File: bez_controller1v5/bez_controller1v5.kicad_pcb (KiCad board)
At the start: 4 copper layers, 100 x 60 mm, 80 parts, among them J1 Conn_01x03_Male, J10 Conn_01x07_Socket, J11 Conn_01x03_Male, J12 Conn_01x03_Male, J13 USB_B_Mini, J14 JTAG Conn_01x06_Male, J15 IMU Conn_01x08_Female, J2 Conn_01x03_Male, J3 Conn_01x03_Male, J4 Screw_Terminal_01x02, J5 Conn_01x03_Male, J6 Conn_01x03_Male, J7 Conn_01x03_Male, J8 JTAG Conn_01x06_Male, J9 Conn_01x09_Socket, U1 PX07806-500-S, U10 USBLC6-4SC6, U11 74LVC2G241, U12 74LVC2G241, U2 74LVC2G241, U3 74LVC2G241, U4 LF50ABV_TO220, U5 LD1117AS33TR_SOT223, U6 INA180A1, U7 STM32F446RETx, U8 74LVC2G241, U9 74LVC2G241, Y1 8MHz

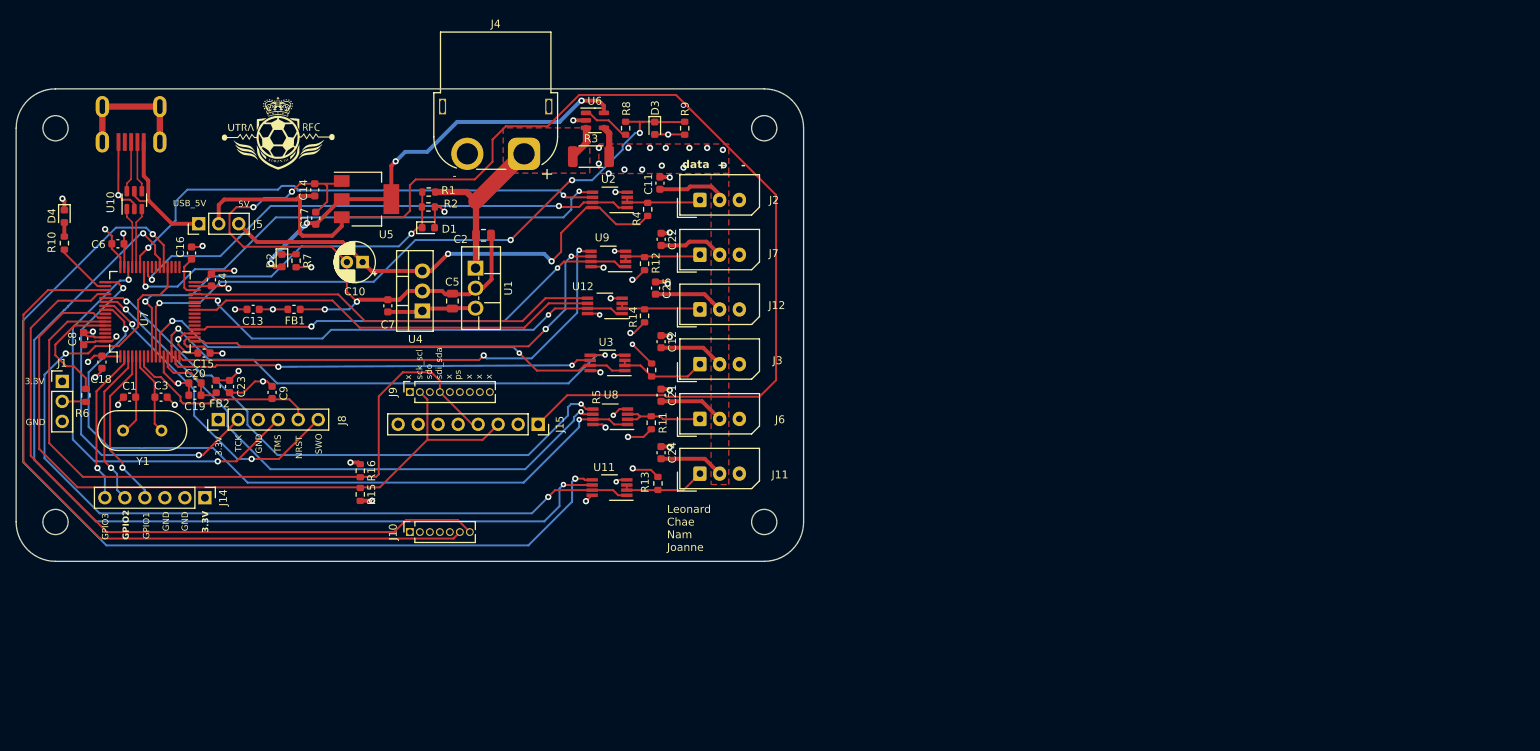
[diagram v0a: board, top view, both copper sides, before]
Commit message: First iteration of the new board with new functions
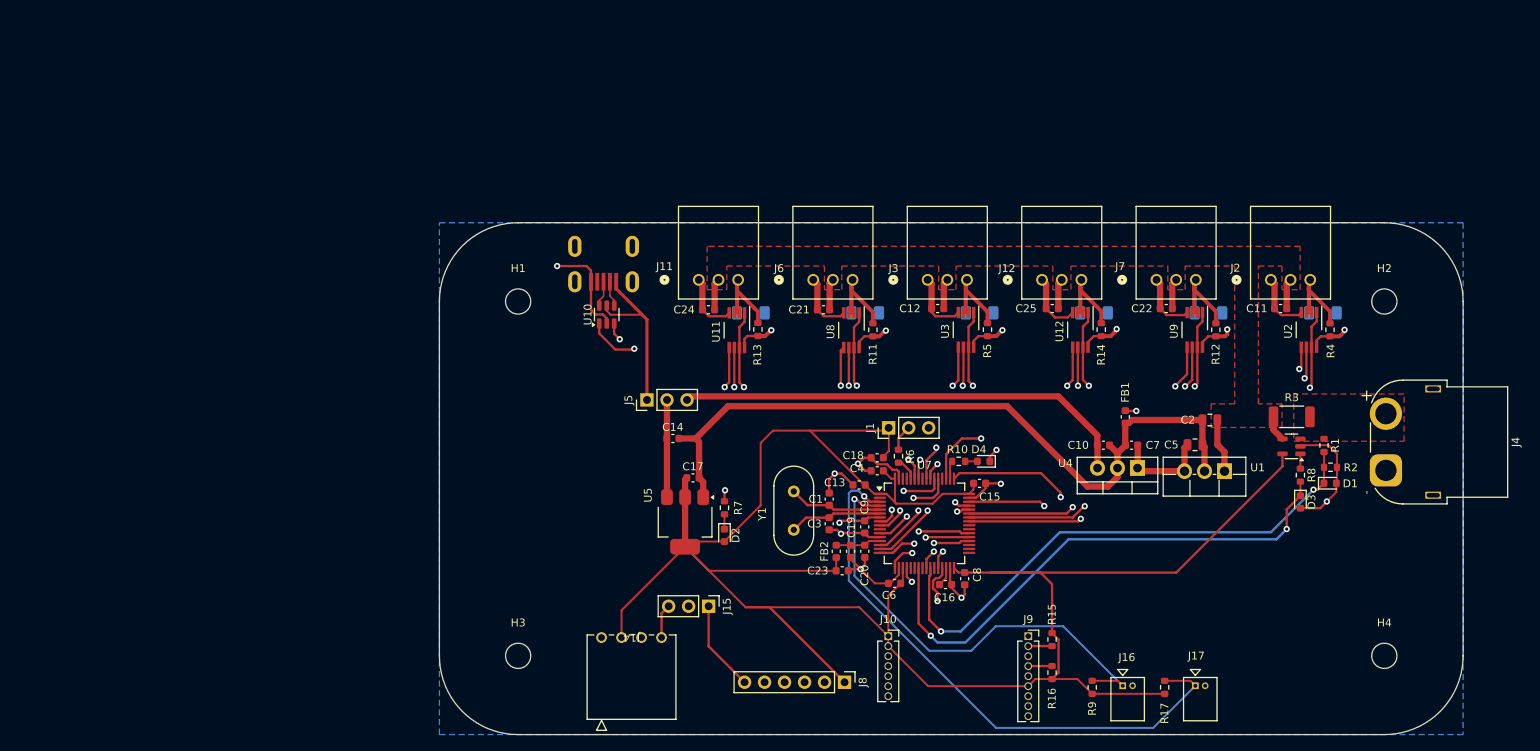
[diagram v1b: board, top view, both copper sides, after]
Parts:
- removed G***: LOGO, LOGO
- added D10: BZV55B5V1, Diode_SMD:D_MiniMELF, B.Cu at (181.4, 54.5)
- added D5: BZV55B5V1, Diode_SMD:D_MiniMELF, B.Cu at (166.9, 54.5)
- added D6: BZV55B5V1, Diode_SMD:D_MiniMELF, B.Cu at (123.3, 54.5)
- added D7: BZV55B5V1, Diode_SMD:D_MiniMELF, B.Cu at (195.9, 54.5)
- added D8: BZV55B5V1, Diode_SMD:D_MiniMELF, B.Cu at (137.8, 54.5)
- added D9: BZV55B5V1, Diode_SMD:D_MiniMELF, B.Cu at (152.3, 54.5)
- added J16: MOLEX_Conn_Button, KiCad:CON_530480210_MOL, F.Cu at (170.5, 101.8)
- added J17: MOLEX_Conn_Button, KiCad:CON_530480210_MOL, F.Cu at (179.8, 101.8)
- added R17: 1k, Resistor_SMD:R_0603_1608Metric, F.Cu at (175.8, 102.0)
- C10: footprint Capacitor_THT:CP_Radial_D5.0mm_P2.00mm -> Capacitor_SMD:C_0603_1608Metric
- J11, J12, J2, J3, J6, J7: footprint Connector_Molex:Molex_SPOX_5267-03A_1x03_P2.50mm_Vertical -> KiCad:CONN_S3B-XH-ALFSN_JST
- J13: footprint USB-Library:USB_MINI -> KiCad:USB_MINI
- J14: value JTAG Conn_01x06_Male -> PPTC041LGBN-RC; footprint Connector_PinHeader_2.54mm:PinHeader_1x06_P2.54mm_Vertical -> KiCad:CONN_PPTC041LGBN-RC_SUL
- J15: value IMU Conn_01x08_Female -> Conn_01x03_Male; footprint Connector_PinSocket_2.54mm:PinSocket_1x08_P2.54mm_Vertical -> Connector_PinHeader_2.54mm:PinHeader_1x03_P2.54mm_Vertical
- R3: value 5m -> 10m
- R9: value 10k -> 1k
- U11, U12, U2, U3, U8, U9: footprint Package_SO:VSSOP-8_3.0x3.0mm_P0.65mm -> KiCad:VSSOP-8_3.0x3.0mm_P0.65mm
- moved H2 170.2 mm to (203.8, 53.0)
- moved D4 120.8 mm to (152.9, 73.3), turned to 180 degrees
- moved R2 119.2 mm to (196.9, 74.0)
- moved D1 119.0 mm to (196.9, 76.1)
- moved R1 118.2 mm to (196.1, 71.3), turned to -90 degrees
- moved R10 116.9 mm to (149.7, 73.3), turned to 180 degrees
- moved J4 116.6 mm to (203.9, 74.5), turned to -90 degrees
- moved C8 116.0 mm to (150.4, 88.2), turned to -90 degrees
- moved C6 107.6 mm to (141.6, 88.8), turned to 180 degrees
- moved FB1 106.4 mm to (170.8, 67.7), turned to -90 degrees
- moved J1 105.1 mm to (140.8, 69.0), turned to 90 degrees
- moved C16 104.6 mm to (148.0, 89.0), turned to 0 degrees
- moved R6 103.5 mm to (142.1, 72.7), turned to -90 degrees
- moved H4 103.4 mm to (203.8, 98.0)
- moved U7 102.0 mm to (145.3, 81.2), turned to 0 degrees
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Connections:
- C11 pad 2: +12V -> /post_shunt_12v
- C12 pad 2: +12V -> /post_shunt_12v
- C2 pad 1: +12V -> /post_shunt_12v
- C21 pad 2: +12V -> /post_shunt_12v
- C22 pad 2: +12V -> /post_shunt_12v
- C24 pad 2: +12V -> /post_shunt_12v
- C25 pad 2: +12V -> /post_shunt_12v
- J11 pad 2: +12V -> /post_shunt_12v
- J12 pad 2: +12V -> /post_shunt_12v
- J14 pad 1: +3.3V -> GND
- J14 pad 2: GND -> +3.3V
- J14 pad 3: GND -> /Screen_SCL
- J14 pad 4: /GPIO1 -> /Screen_SDA
- J15 pad 1: /power -> /SWO
- J15 pad 2: GND -> /SWO_or_Screen_SDA
- J15 pad 3: /SCK_SCL -> /Screen_SDA
- J2 pad 2: +12V -> /post_shunt_12v
- J3 pad 2: +12V -> /post_shunt_12v
- J6 pad 2: +12V -> /post_shunt_12v
- J7 pad 2: +12V -> /post_shunt_12v
- R3 pad 2: +12V -> /post_shunt_12v
- R9 pad 1: /V_shunt_read -> +3.3V
- R9 pad 2: GND -> /GPIO1
- U1 pad 1: +12V -> /post_shunt_12v
- U6 pad 4: +12V -> /post_shunt_12v
- U7 pad 10: /V_shunt_read -> unconnected-(U7-PC2-Pad10)
- U7 pad 2: /GPIO3 -> unconnected-(U7-PC13-Pad2)
- U7 pad 23: unconnected-(U7-PA7-Pad23) -> /V_shunt_read
- U7 pad 26: unconnected-(U7-PB0-Pad26) -> /V_bat_read
- U7 pad 29: /USART3_TX -> /Screen_SCL
- U7 pad 51: /INT1 -> /USART3_TX
- U7 pad 52: /INT2 -> unconnected-(U7-PC11-Pad52)
- U7 pad 55: /SWO -> /SWO_or_Screen_SDA
- U7 pad 8: unconnected-(U7-PC0-Pad8) -> /INT1
- U7 pad 9: /V_bat_read -> /INT2
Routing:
- net +3.3V: track 90.1 -> 283.7 mm, vias 13 -> 0
- net /power: track 153.5 -> 12.3 mm
- net +12V: track 82.2 -> 0.00 mm, vias 14 -> 0
- net /USART6_TX: track 126.1 -> 48.4 mm
- net /USART6_RX: track 117.2 -> 48.2 mm
- net /USART6_DIR: track 113.7 -> 48.0 mm
- net /INT1: track 90.2 -> 25.9 mm, vias 0 -> 1
- net /Screen_SCL: track 0.00 -> 61.3 mm, vias 0 -> 1
- net /INT2: track 88.5 -> 27.8 mm, vias 0 -> 1
- net /USART5_DIR: track 94.3 -> 34.9 mm
- net /SCK_SCL: track 94.2 -> 35.5 mm, vias 0 -> 1
- net /USB_D-: track 7.65 -> 64.9 mm, vias 0 -> 2
- net /USB_D+: track 7.64 -> 63.4 mm, vias 0 -> 2
- net /GPIO2: track 20.3 -> 73.9 mm
- net /SDI_SDA: track 92.3 -> 39.2 mm, vias 0 -> 1
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- added copper zone on F.Cu, net /post_shunt_12v
- added copper zone on B.Cu, net GND
- removed copper zone on In1.Cu, net +12V
- removed copper zone on In1.Cu, net +3.3V
- removed copper zone on In2.Cu, net GND
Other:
- board size 100 x 60 mm -> 130 x 65 mm
- board text removed: "+"
- board text removed: "-"
- board text removed: "3.3V"
- board text removed: "5V"
- board text removed: "GND"
- board text removed: "GPIO1"
- board text removed: "GPIO2"
- board text removed: "GPIO3"
- board text removed: "Leonard Chae Nam Joanne"
- board text removed: "NRST"
- board text removed: "SWO"
- board text removed: "TCK"
- board text removed: "TMS"
- board text removed: "USB_5V"
- board text removed: "data"
- board text removed: "ps"
- board text removed: "sck_scl"
- board text removed: "sdi_sda"
- board text removed: "sdo"
- board text removed: "x"
